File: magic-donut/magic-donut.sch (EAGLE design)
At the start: 26 parts

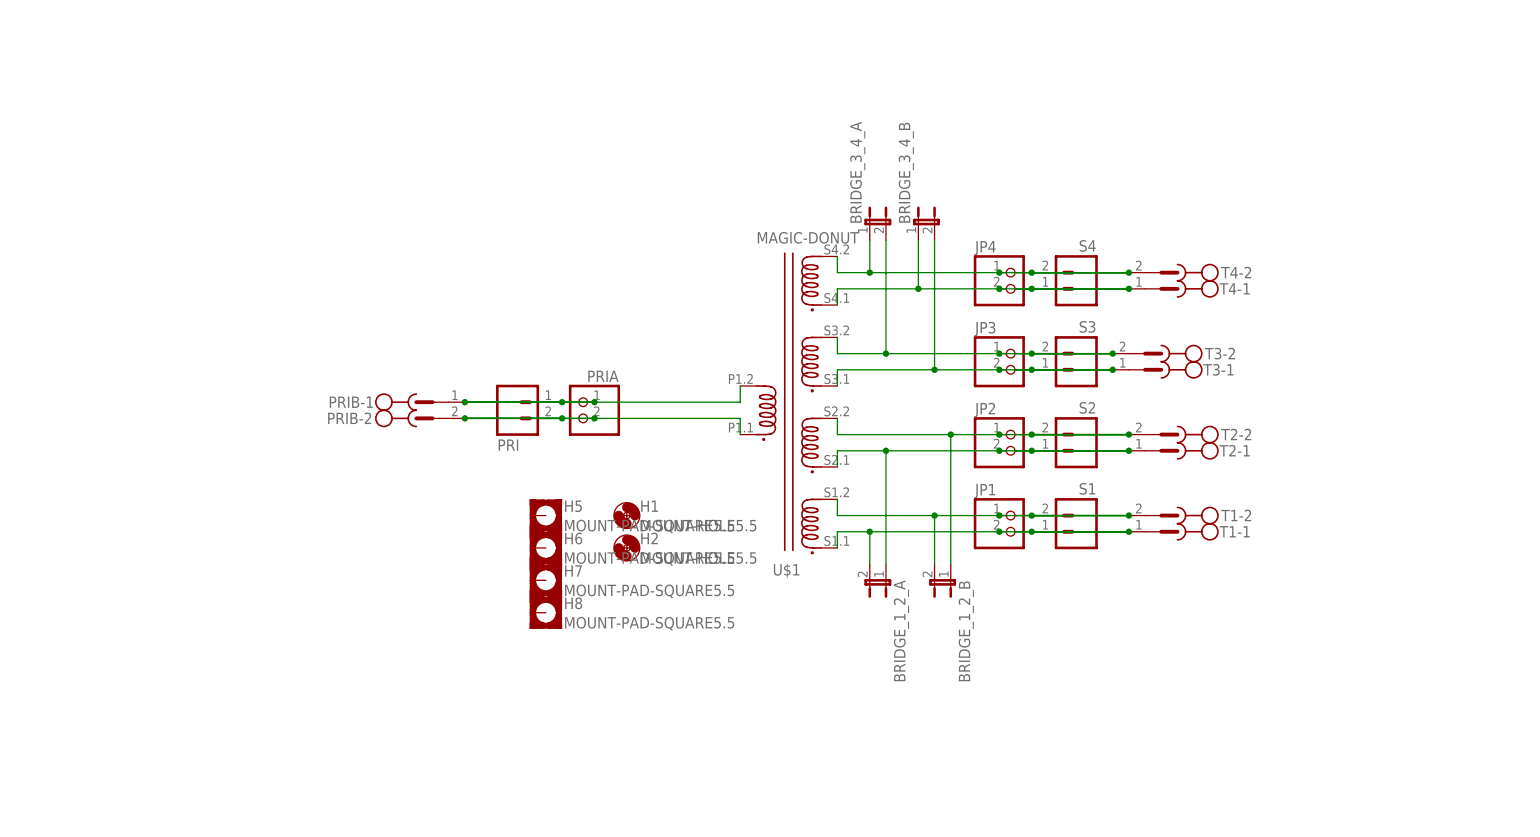
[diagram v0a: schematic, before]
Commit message: WIP
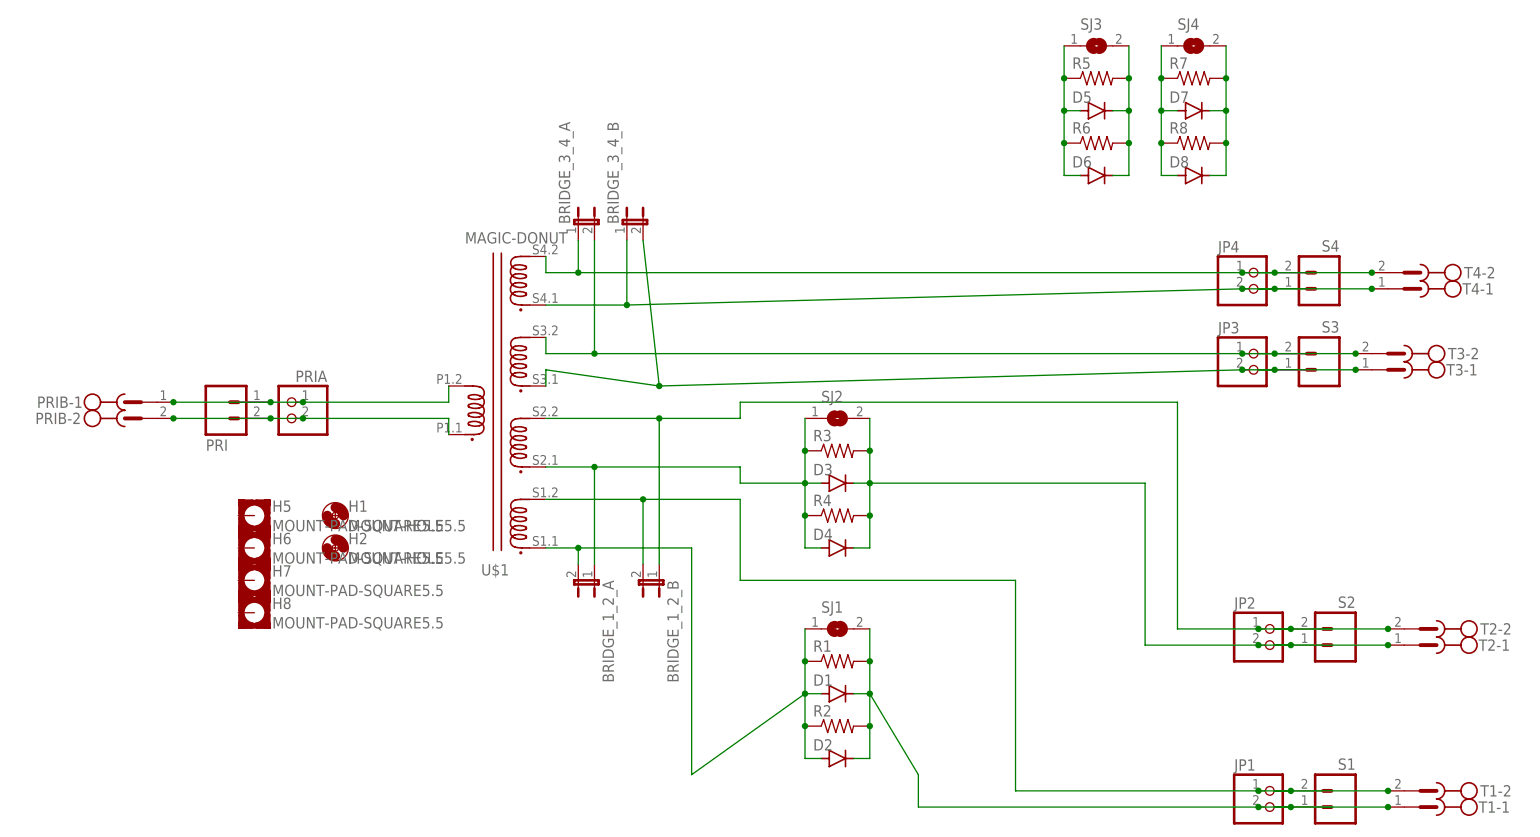
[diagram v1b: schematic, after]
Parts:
- added D1, D3, D5, D7: (no value), diode:DIODE-DO214AA
- added D2, D4, D6, D8: (no value), diode:DIODE-DO201-15
- added R1, R3, R5, R7: (no value), rcl:R-US_R0805
- added R2, R4, R6, R8: (no value), rcl:R-US_0207/2V
- added SJ1, SJ2, SJ3, SJ4: (no value), jumper:SJ
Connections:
- removed net N$2 (its old number): BRIDGE_1_2_A.1, JP2.2, S2.1, T2-1.SK, U$1.S2.1
- new net N$13: D1.C, D2.C, JP1.2, R1.2, R2.2, S1.1, SJ1.2, T1-1.SK
- new net N$16: D3.C, D4.C, JP2.2, R3.2, R4.2, S2.1, SJ2.2, T2-1.SK
- new net N$17: D5.A, D6.A, R5.1, R6.1, SJ3.1
- new net N$18: D5.C, D6.C, R5.2, R6.2, SJ3.2
- new net N$19: D7.A, D8.A, R7.1, R8.1, SJ4.1
- new net N$20: D7.C, D8.C, R7.2, R8.2, SJ4.2
- new net N$8: BRIDGE_1_2_A.1, D3.A, D4.A, R3.1, R4.1, SJ2.1, U$1.S2.1
- net N$1: now also D1.A, D2.A, R1.1, R2.1, SJ1.1; no longer JP1.2, S1.1, T1-1.SK
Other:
- moved on the sheet: BRIDGE_1_2_A, BRIDGE_1_2_B, BRIDGE_3_4_A, BRIDGE_3_4_B, H1, H2, H5, H6, H7, H8, JP1, JP2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
